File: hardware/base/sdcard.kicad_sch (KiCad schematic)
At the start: 3 parts, among them J1 MEM2067

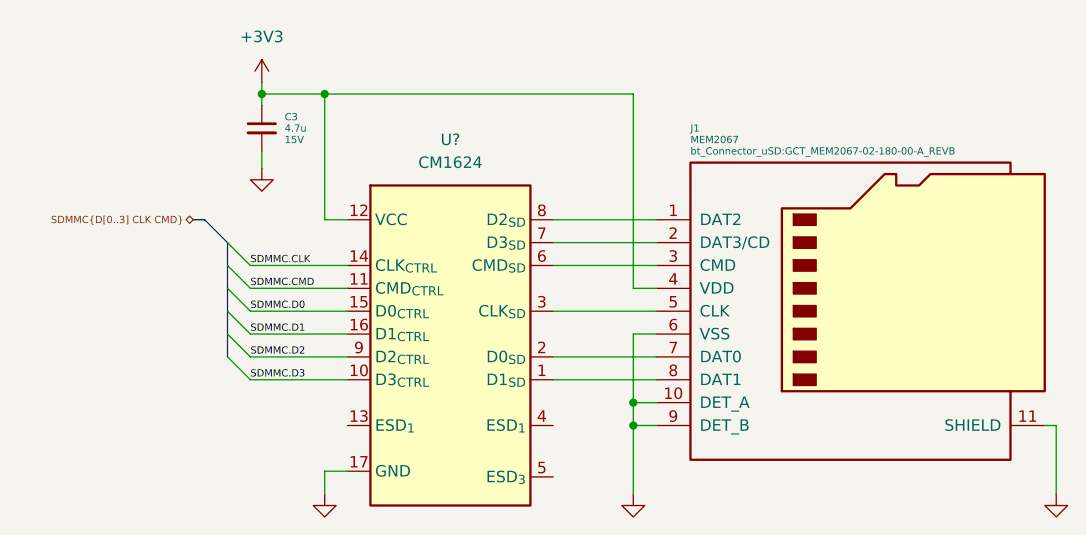
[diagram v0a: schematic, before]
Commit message: schematic complete unreviewed
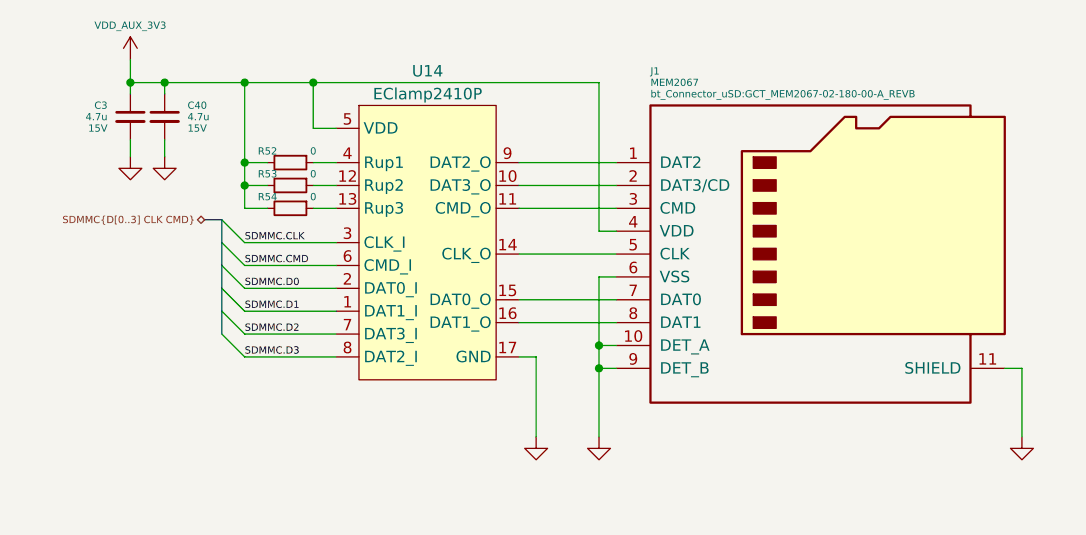
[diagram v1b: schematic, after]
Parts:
- removed U?: CM1624, symbol bt_Protection:CM1624
- added C40: 4.7u, Capacitor_SMD:C_0603_1608Metric, symbol Device:C_Small
- added R52, R53, R54: 0, Resistor_SMD:R_0402_1005Metric, symbol Device:R_Small
- added U14: EClamp2410P, bt_Package_DFN:UDFN-16-4x1.6_P0.5mm_EP3x0.5mm, symbol bt_Protection:EClamp2410P
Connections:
- net GND: now also C40.2, U14.17 (GND)
- net SDMMC.CLK: now also U14.3 (CLK_I)
- net SDMMC.CMD: now also U14.6 (CMD_I)
- net SDMMC.D0: now also U14.2 (DAT0_I)
- net SDMMC.D1: now also U14.1 (DAT1_I)
- net SDMMC.D2: now also U14.7 (DAT3_I)
- net SDMMC.D3: now also U14.8 (DAT2_I)
- net at J1.8 (DAT1): now also U14.16 (DAT1_O)
- net at J1.7 (DAT0): now also U14.15 (DAT0_O)
- net at J1.5 (CLK): now also U14.14 (CLK_O)
- net at J1.3 (CMD): now also U14.11 (CMD_O)
- net at J1.2 (DAT3/CD): now also U14.10 (DAT3_O)
- net at J1.1 (DAT2): now also U14.9 (DAT2_O)
- net +3V3 renamed VDD_AUX_3V3
- net VDD_AUX_3V3: now also C40.1, R52.2, R53.2, R54.2, U14.5 (VDD)
- new net: R52.1, U14.4 (Rup1)
- new net: R53.1, U14.12 (Rup2)
- new net: R54.1, U14.13 (Rup3)
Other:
- moved on the sheet: C3
